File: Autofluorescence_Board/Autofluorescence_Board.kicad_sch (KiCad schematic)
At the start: 14 parts, among them U1 PAM2863ECR

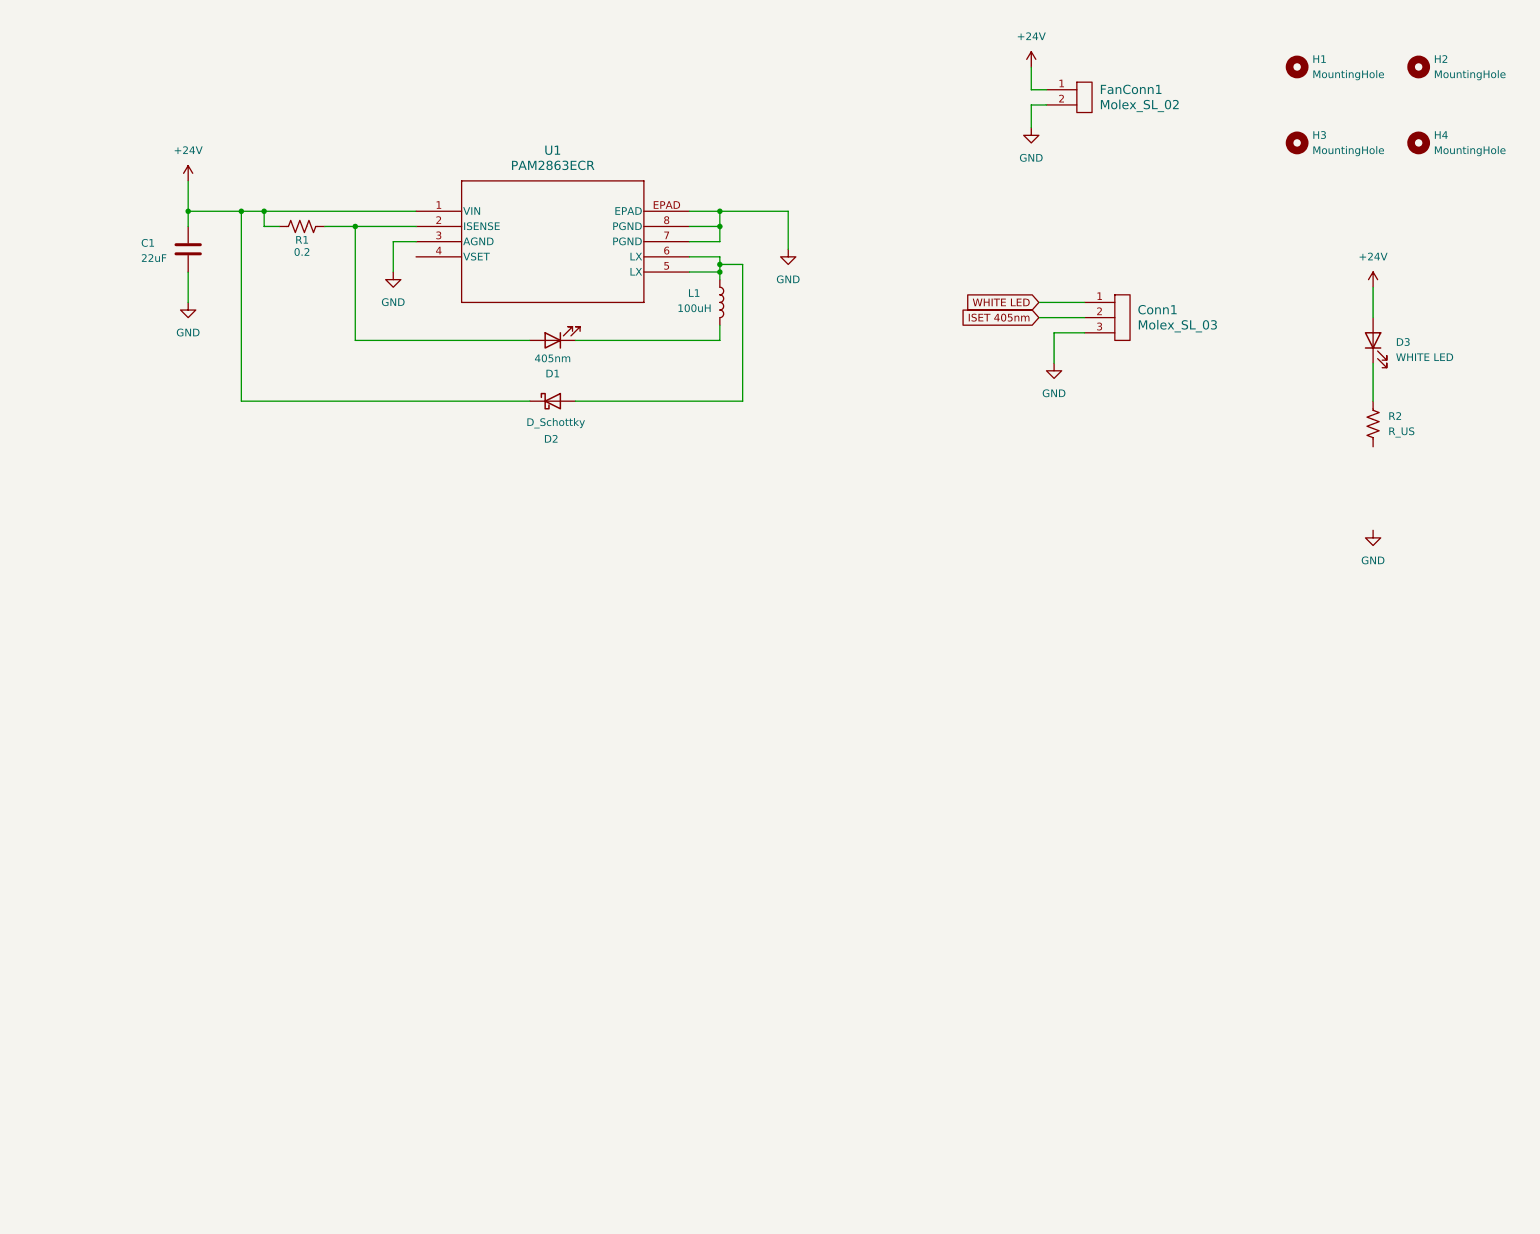
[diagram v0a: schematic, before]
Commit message: Footprints Added, and all the other stuff -morgan
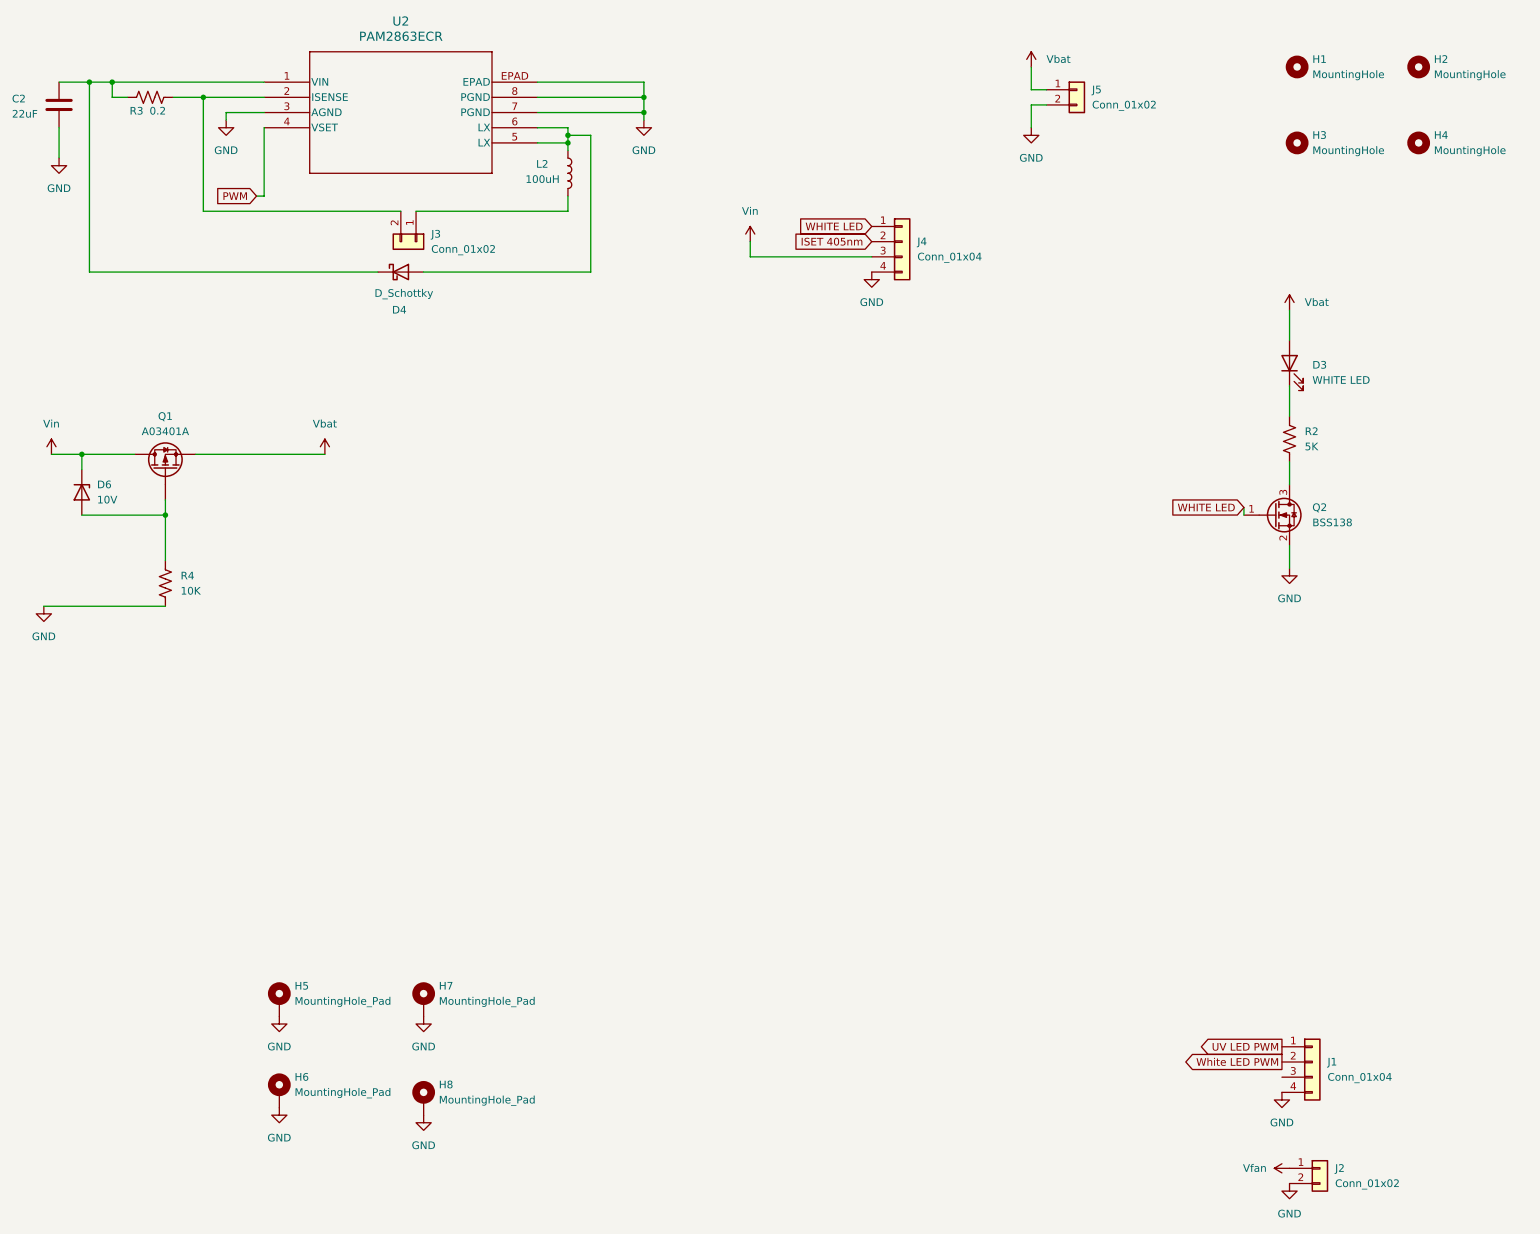
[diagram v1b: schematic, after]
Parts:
- removed C1: 22uF, symbol Device:C
- removed Conn1: Molex_SL_03, symbol MRDT_Connectors:Molex_SL_03
- removed D1: 405nm, symbol Device:LED
- removed D2: D_Schottky, symbol Device:D_Schottky
- removed FanConn1: Molex_SL_02, symbol MRDT_Connectors:Molex_SL_02
- removed L1: 100uH, symbol Device:L
- removed R1: 0.2, symbol Device:R_US
- removed U1: PAM2863ECR, SOIC_863ECR_DIO, symbol AF_SymbolLibrary:PAM2863ECR
- added C2: 22uF, Capacitor_SMD:C_0603_1608Metric_Pad1.08x0.95mm_HandSolder, symbol Device:C
- added D4: D_Schottky, Diode_SMD:D_SOD-123, symbol Device:D_Schottky
- added D6: 10V, Package_DIP:DIP-40_W15.24mm, symbol Device:D_Zener
- added H5, H6, H7, H8: MountingHole_Pad, Package_DFN_QFN:Nordic_AQFN-94-1EP_7x7mm_P0.4mm, symbol Mechanical:MountingHole_Pad
- added J1: Conn_01x04, Package_DFN_QFN:QFN-20-1EP_5x5mm_P0.65mm_EP3.35x3.35mm, symbol Connector_Generic:Conn_01x04
- added J2, J3, J5: Conn_01x02, Package_DFN_QFN:QFN-20-1EP_5x5mm_P0.65mm_EP3.35x3.35mm, symbol Connector_Generic:Conn_01x02
- added J4: Conn_01x04, symbol Connector_Generic:Conn_01x04
- added L2: 100uH, Inductor_SMD:L_0201_0603Metric_Pad0.64x0.40mm_HandSolder, symbol Device:L
- added Q1: A03401A, Package_TO_SOT_SMD:SOT-23, symbol Device:Q_PMOS
- added Q2: BSS138, Package_TO_SOT_SMD:SOT-23, symbol Transistor_FET:BSS138
- added R3: 0.2, Resistor_SMD:R_0603_1608Metric_Pad0.98x0.95mm_HandSolder, symbol Device:R_US
- added R4: 10K, Resistor_SMD:R_0603_1608Metric_Pad0.98x0.95mm_HandSolder, symbol Device:R_US
- added U2: PAM2863ECR, Package_SO:Diodes_SO-8EP, symbol AF_SymbolLibrary:PAM2863ECR
- D3: footprint (none) -> Diode_SMD:D_0603_1608Metric_Pad1.05x0.95mm_HandSolder
- R2: value R_US -> 5K; footprint (none) -> Resistor_SMD:R_0603_1608Metric_Pad0.98x0.95mm_HandSolder
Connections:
- net GND: now also C2.2, H5.1, H6.1, H7.1, H8.1, J1.4 (Pin_4), J2.2 (Pin_2), J4.4 (Pin_4), J5.2 (Pin_2), Q2.2 (S), R4.2, U2.3 (AGND), U2.7 (PGND), U2.8 (PGND), U2.EPAD
- net ISET 405nm: now also J4.2 (Pin_2)
- net WHITE LED: now also J4.1 (Pin_1), Q2.1 (G)
- net at R2.2: now also Q2.3 (D)
- net +24V renamed Vbat
- net Vbat: now also J5.1 (Pin_1), Q1.S
- new net: C2.1, D4.1 (K), R3.1, U2.1 (VIN)
- new net: J3.2 (Pin_2), R3.2, U2.2 (ISENSE)
- new net: D4.2 (A), L2.1, U2.5 (LX), U2.6 (LX)
- new net: D6.2 (A), Q1.G, R4.1
- new net: J3.1 (Pin_1), L2.2
- new net PWM: U2.4 (VSET)
- new net UV LED PWM: J1.1 (Pin_1)
- new net Vfan: J2.1 (Pin_1)
- new net Vin: D6.1 (K), J4.3 (Pin_3), Q1.D
- new net White LED PWM: J1.2 (Pin_2)
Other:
- moved on the sheet: D3, R2
